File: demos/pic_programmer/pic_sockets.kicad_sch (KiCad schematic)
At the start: 7 parts, among them P2 SUPP28, P3 SUPP40, U1 24Cxx, U5 PIC_18_PINS, U6 PIC_8_PINS

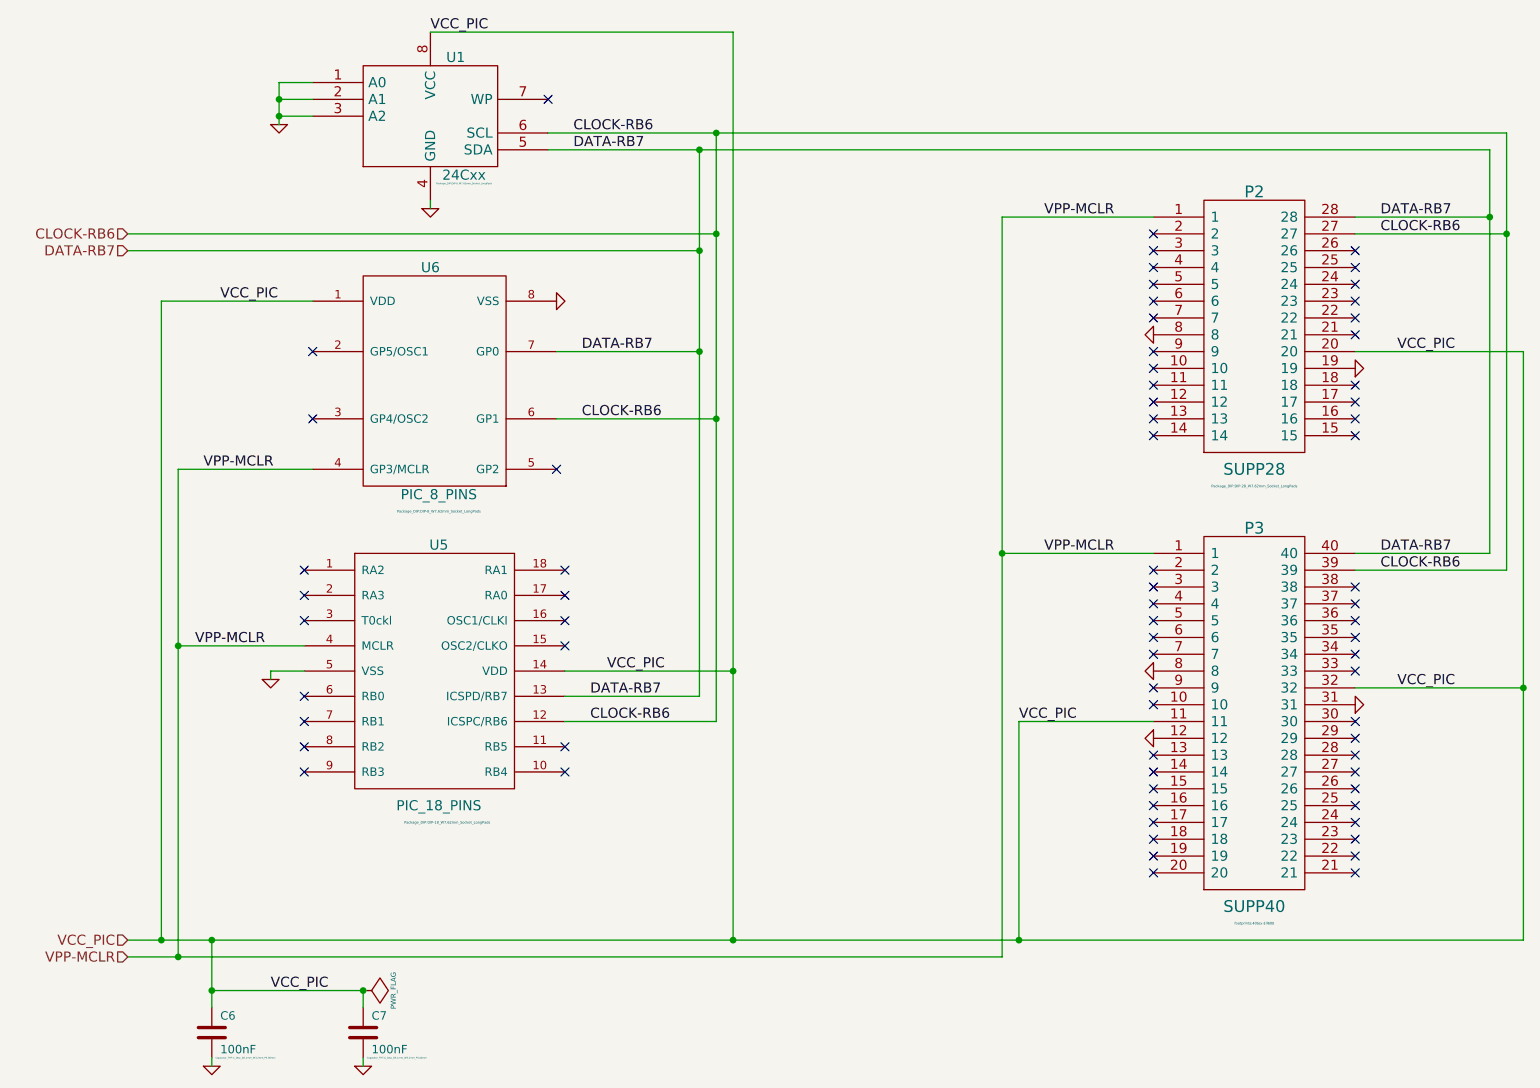
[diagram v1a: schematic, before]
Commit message: Update demos.
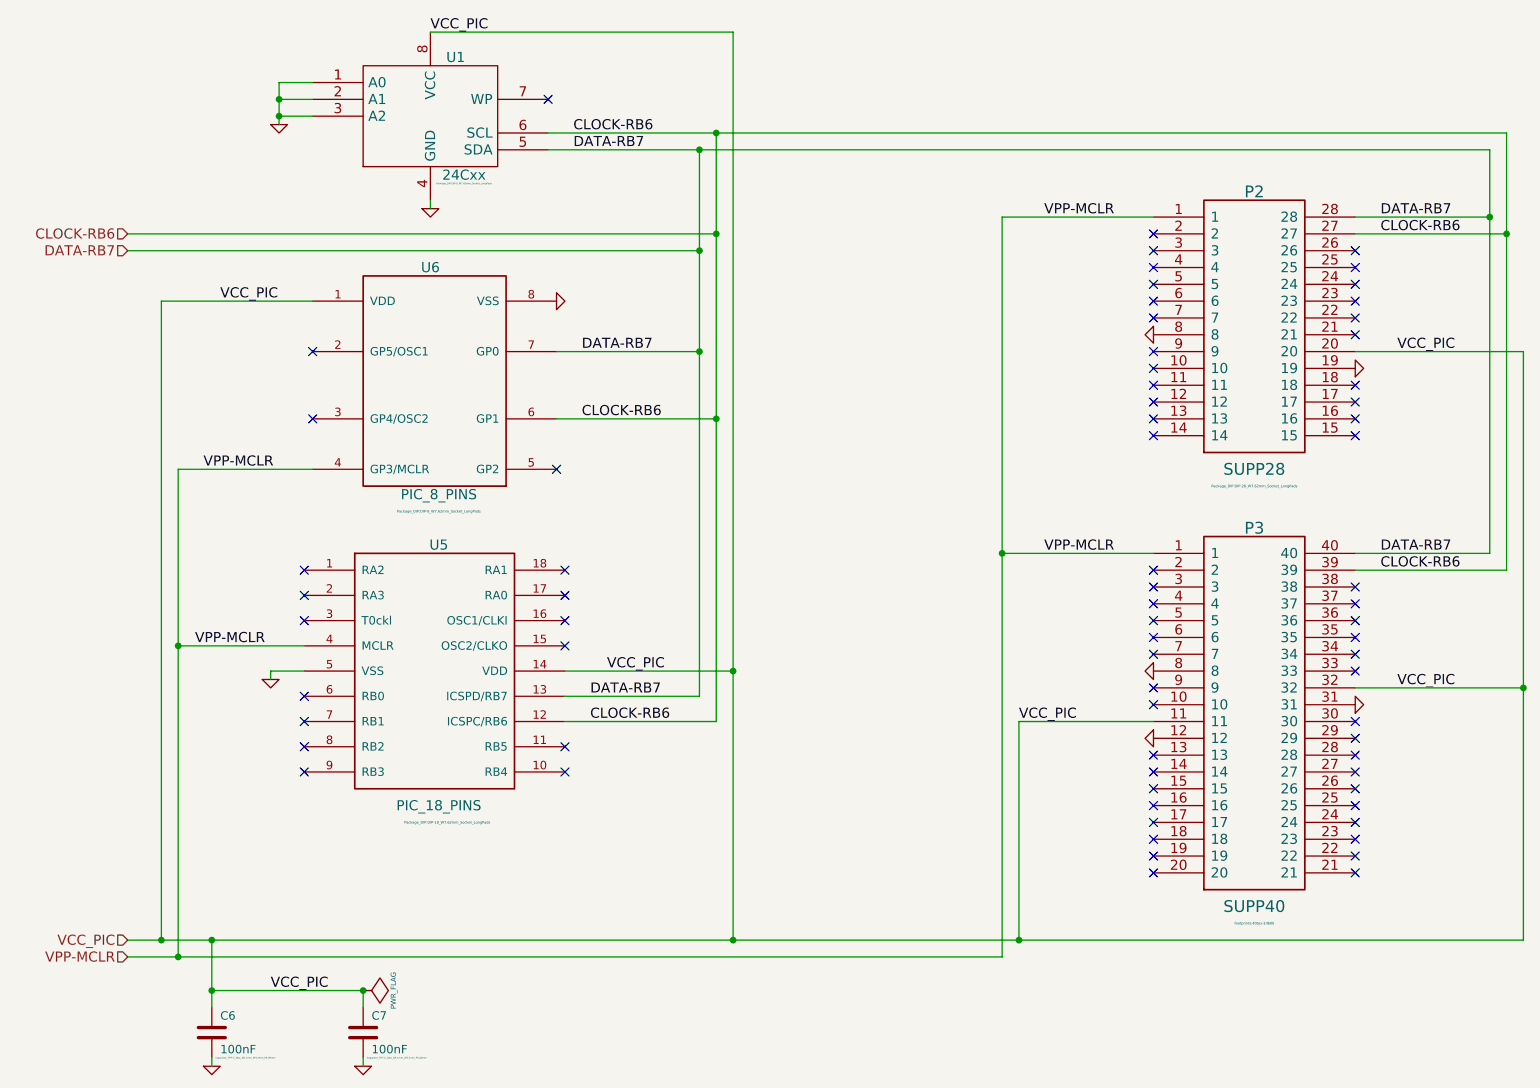
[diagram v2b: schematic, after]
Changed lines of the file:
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@@
-(kicad_sch (version 20210126) (generator eeschema)
+(kicad_sch (version 20210406) (generator eeschema)
   (paper "A4")
   (title_block
@@
       (effects (font (size 1.524 1.524)) hide)
     )
+    (pin "4")
+    (pin "8")
     (pin "1")
     (pin "2")
@@
     (pin "6")
     (pin "7")
-    (pin "4")
-    (pin "8")
   )
   (symbol (lib_id "pic_programmer_schlib:SUPP28") (at 218.44 64.77 0) (unit 1)
